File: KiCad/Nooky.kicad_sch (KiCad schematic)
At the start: 8 parts, among them J1 USB A Input, J2 VIN (5 - 7VDC), J3 VADJ (2.85VDC), J4 VADJ (2.85VDC), U1 LM317 / LM350 / LM338 Regulat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

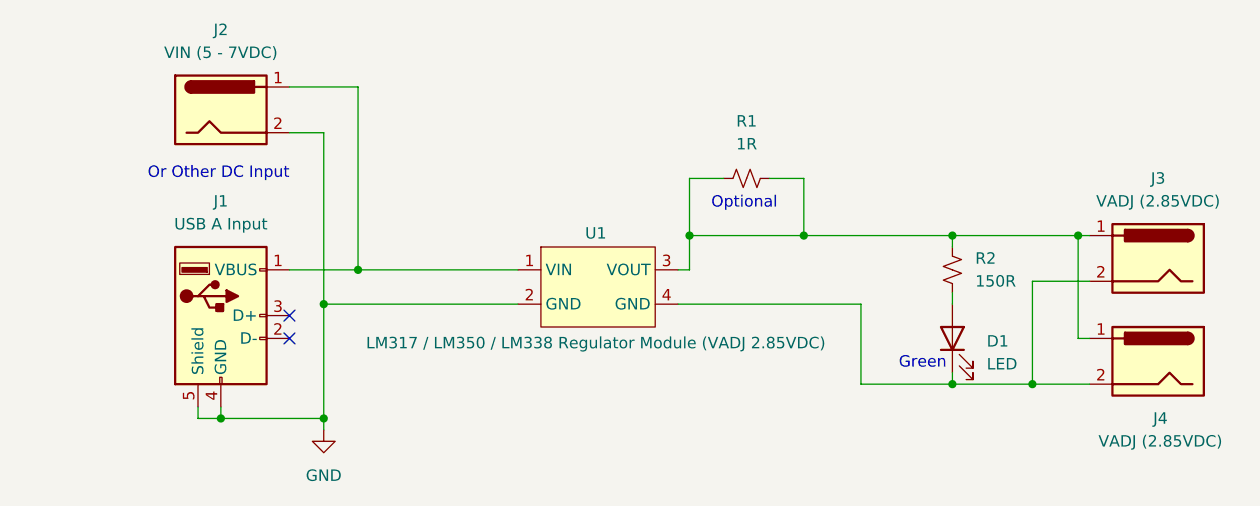
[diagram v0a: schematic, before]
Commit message: Review
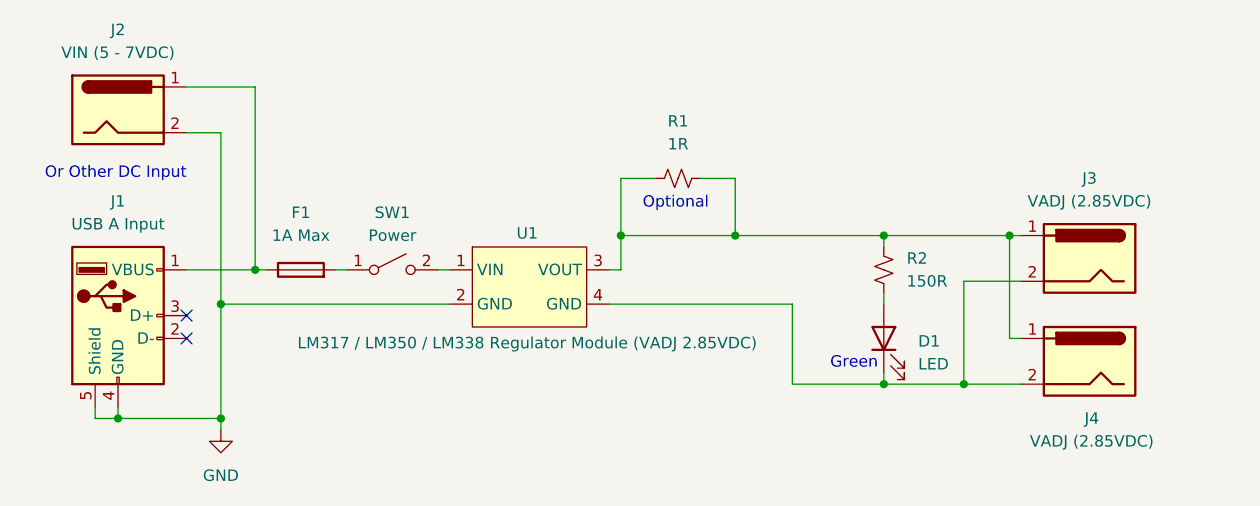
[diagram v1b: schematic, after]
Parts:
- added F1: 1A Max, symbol Device:Fuse
- added SW1: Power, symbol Switch:SW_SPST
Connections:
- net at J1.1 (VBUS), J2.1: now also F1.1; no longer U1.1 (VIN)
- new net: F1.2, SW1.1 (A)
- new net: SW1.2 (B), U1.1 (VIN)
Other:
- moved on the sheet: D1, J1, J2, J3, J4, R1, R2, U1
